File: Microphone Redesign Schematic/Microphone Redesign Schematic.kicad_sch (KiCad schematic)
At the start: 17 parts, among them J1 Custom_3p_2.0MM, U1 ${SIM.PARAMS}

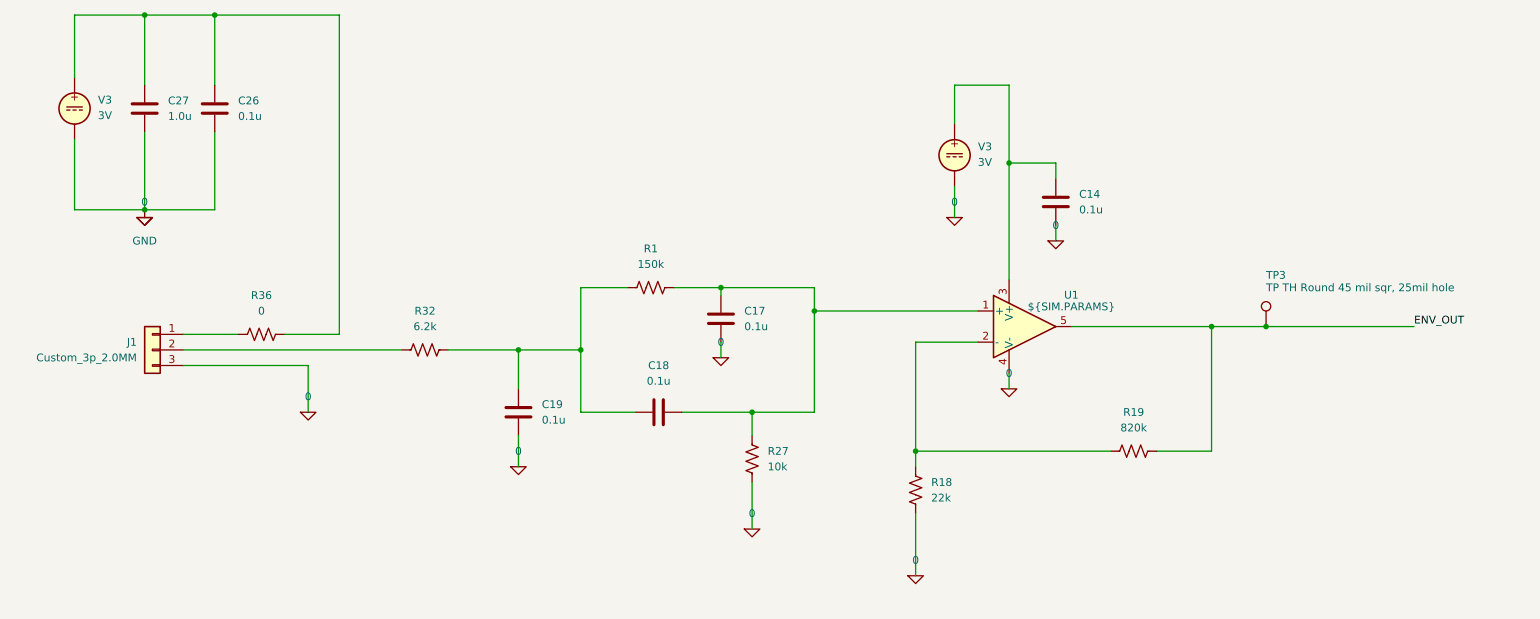
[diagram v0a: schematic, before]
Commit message: updated shcematics after meeting 1/21/26
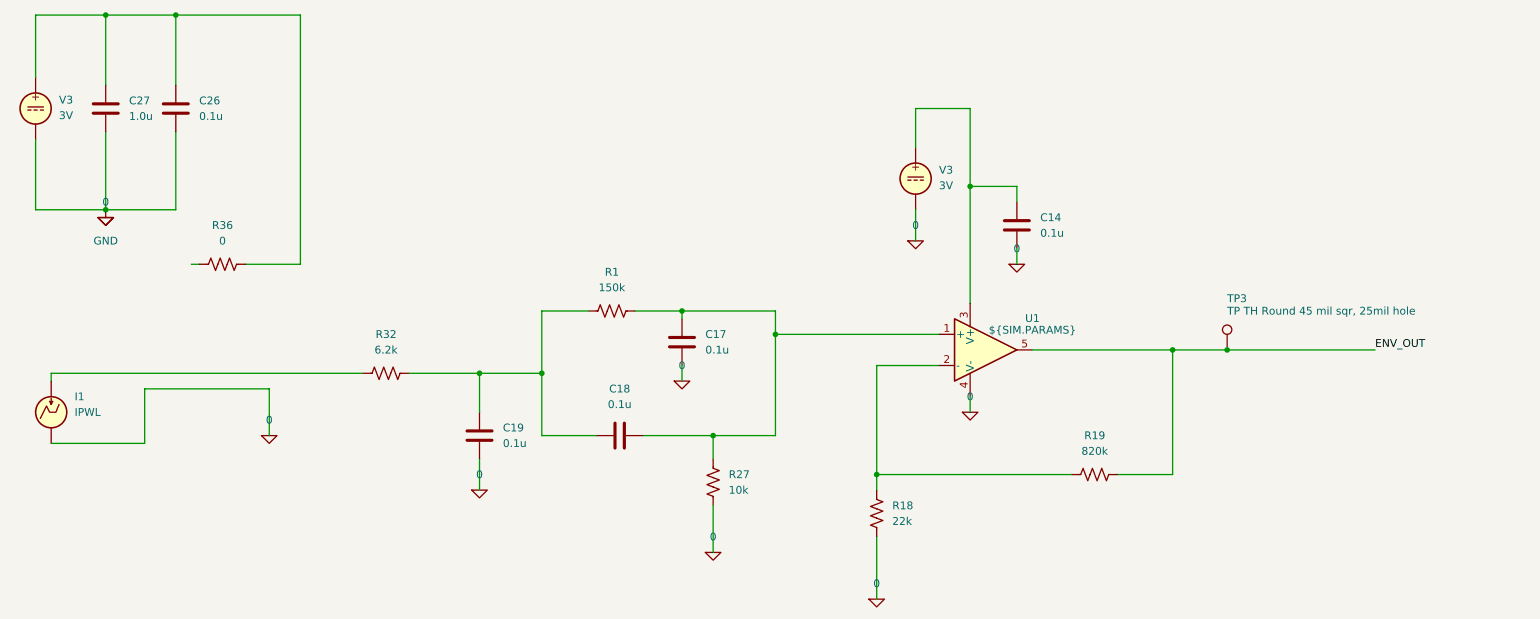
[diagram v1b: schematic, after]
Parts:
- removed J1: Custom_3p_2.0MM, symbol Connector_Generic:Conn_01x03
- added I1: IPWL, symbol Simulation_SPICE:IPWL
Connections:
- net 0: now also I1.2
- net at R32.2: now also I1.1
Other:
- moved on the sheet: C14, C17, C18, C19, C26, C27, R1, R18, R19, R27, R32, R36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
